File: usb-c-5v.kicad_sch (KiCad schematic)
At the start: 10 parts, among them J6 KH-TYPE-C-16P (Kinghelm), U8 AP2112K-3.3

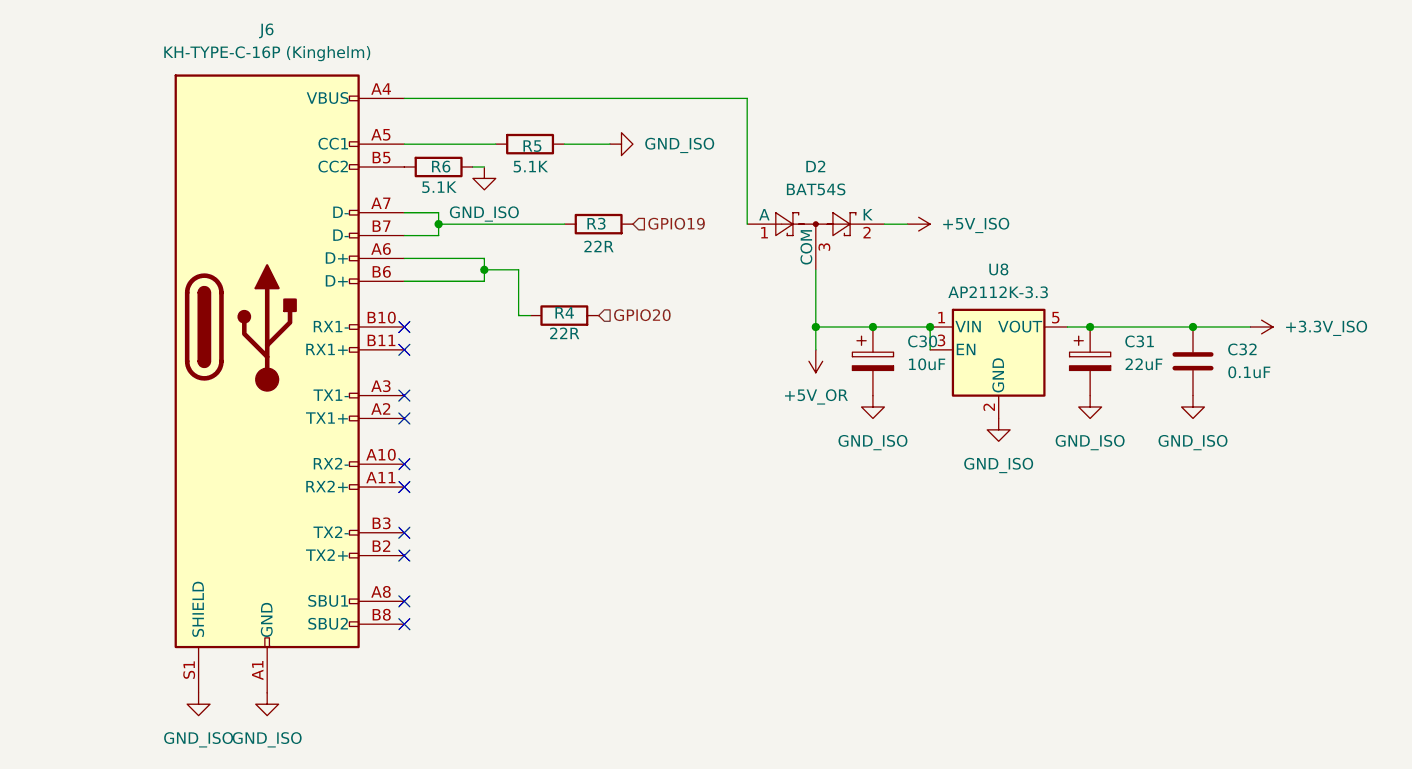
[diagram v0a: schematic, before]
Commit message: Finishing touches
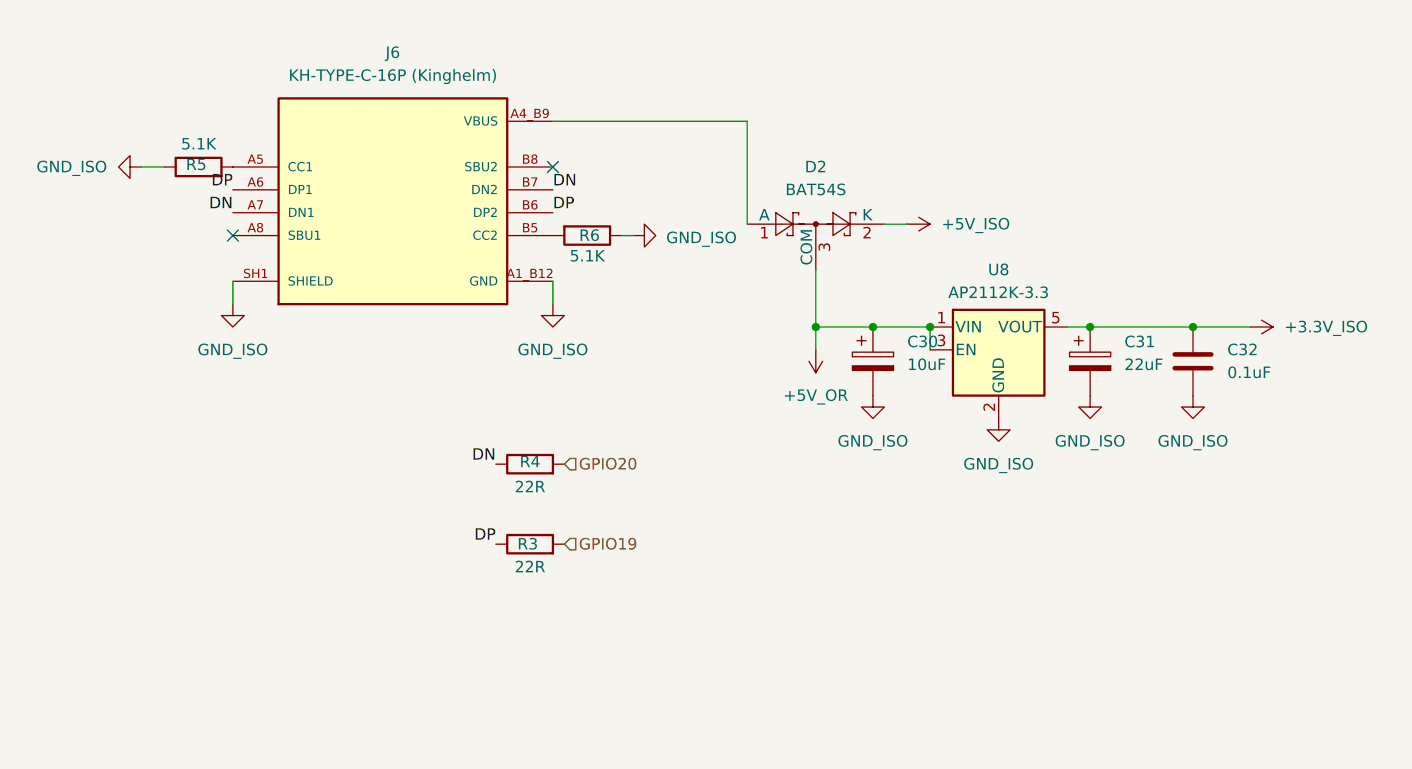
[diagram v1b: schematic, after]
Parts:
- J6: footprint Connector_USB:USB_C_Receptacle_GCT_USB4110 -> KH-TYPE-C-16P:KINGHELM_KH-TYPE-C-16P; symbol Connector:USB_C_Receptacle -> KH-TYPE-C-16P:KH-TYPE-C-16P; Availability (none) -> Not in stock; Check_prices (none) -> https://www.snapeda.com/parts/KH-TYPE-C-16P/Kinghelm/view-p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; MANUFACTURER (none) -> Kinghelm; MAXIMUM_PACKAGE_HEIGHT (none) -> 3.41mm; MF (none) -> kinghelm; MP (none) -> KH-TYPE-C-16P; PARTREV (none) -> A0; Package (none) -> None; Price (none) -> None; SNAPEDA_PN (none) -> KH-TYPE-C-16P; STANDARD (none) -> Manufacturer Recommendations; SnapEDA_Link (none) -> https://www.snapeda.com/parts/KH-TYPE-C-16P/Kinghelm/view-p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
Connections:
- net DN: now reaches J6.A7 (DN1), J6.B7 (DN2)
- net DN: now also R4.1; no longer R3.1
- net DP: now reaches J6.A6 (DP1), J6.B6 (DP2)
- net DP: now also R3.1; no longer R4.1
- net GND_ISO renamed GND
- net GND: now also J6.A12_B1 (GND), J6.A1_B12 (GND), J6.SH1 (SHIELD), J6.SH2 (SHIELD), J6.SH3 (SHIELD), J6.SH4 (SHIELD); no longer J6.A1 (GND), J6.A12 (GND), J6.B1 (GND), J6.B12 (GND), J6.S1 (SHIELD)
- new net VBUS: D2.1 (A), J6.A4_B9 (VBUS), J6.A9_B4 (VBUS)
- no-connect marks 10 -> 2
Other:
- moved on the sheet: R3, R4, R5, R6
